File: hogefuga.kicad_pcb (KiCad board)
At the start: 2 copper layers, 95.3 x 97.6 mm, 45 parts, among them J1 MJ-4PP-9, SW1 SW_PUSH, SW10 SW_PUSH, SW11 SW_PUSH, SW12 SW_PUSH, SW13 SW_PUSH, SW14 SW_PUSH, SW15 SW_PUSH, SW16 SW_PUSH, SW17 SW_PUSH, SW18 SW_PUSH, SW19 SW_PUSH, SW2 SW_PUSH, SW20 SW_PUSH, SW3 SW_PUSH, SW4 SW_PUSH, SW5 SW_PUSH, SW6 SW_PUSH, SW7 SW_PUSH, SW8 SW_PUSH, SW9 SW_PUSH, U1 ProMicro

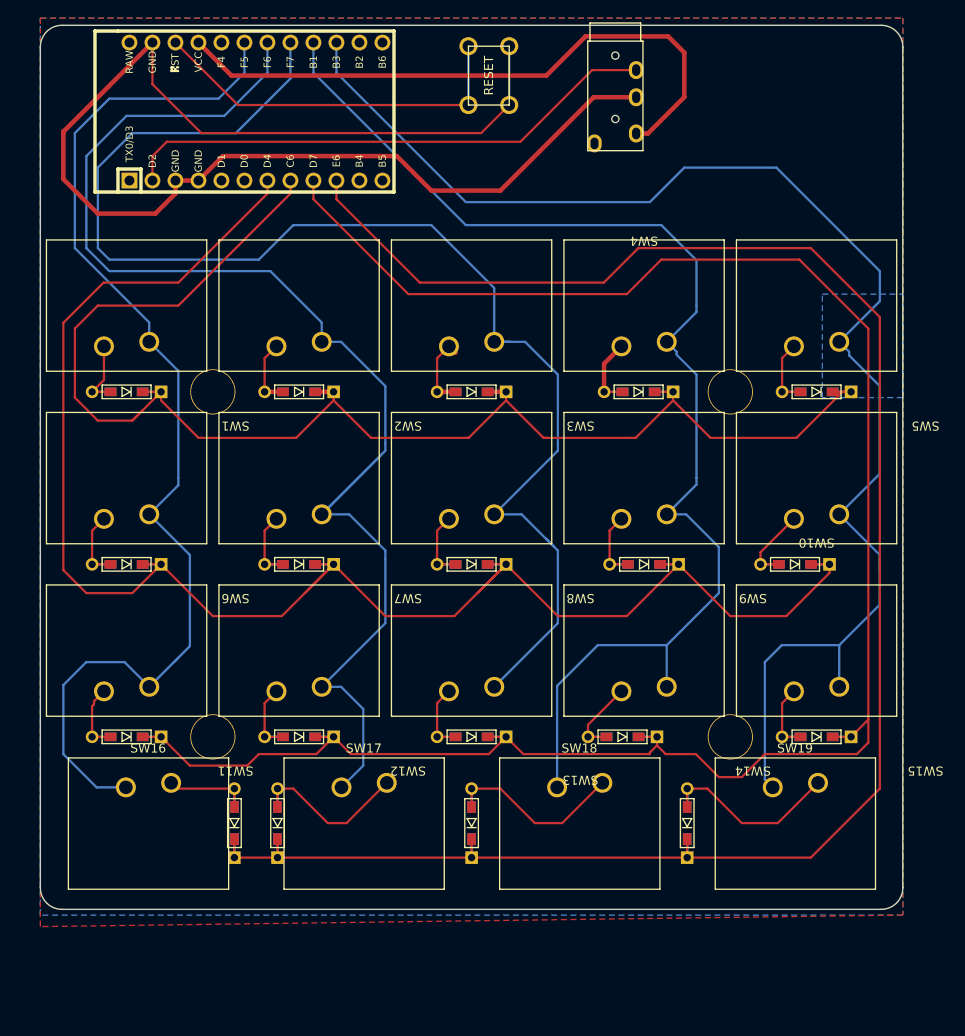
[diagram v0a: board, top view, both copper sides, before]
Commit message: rev0.2
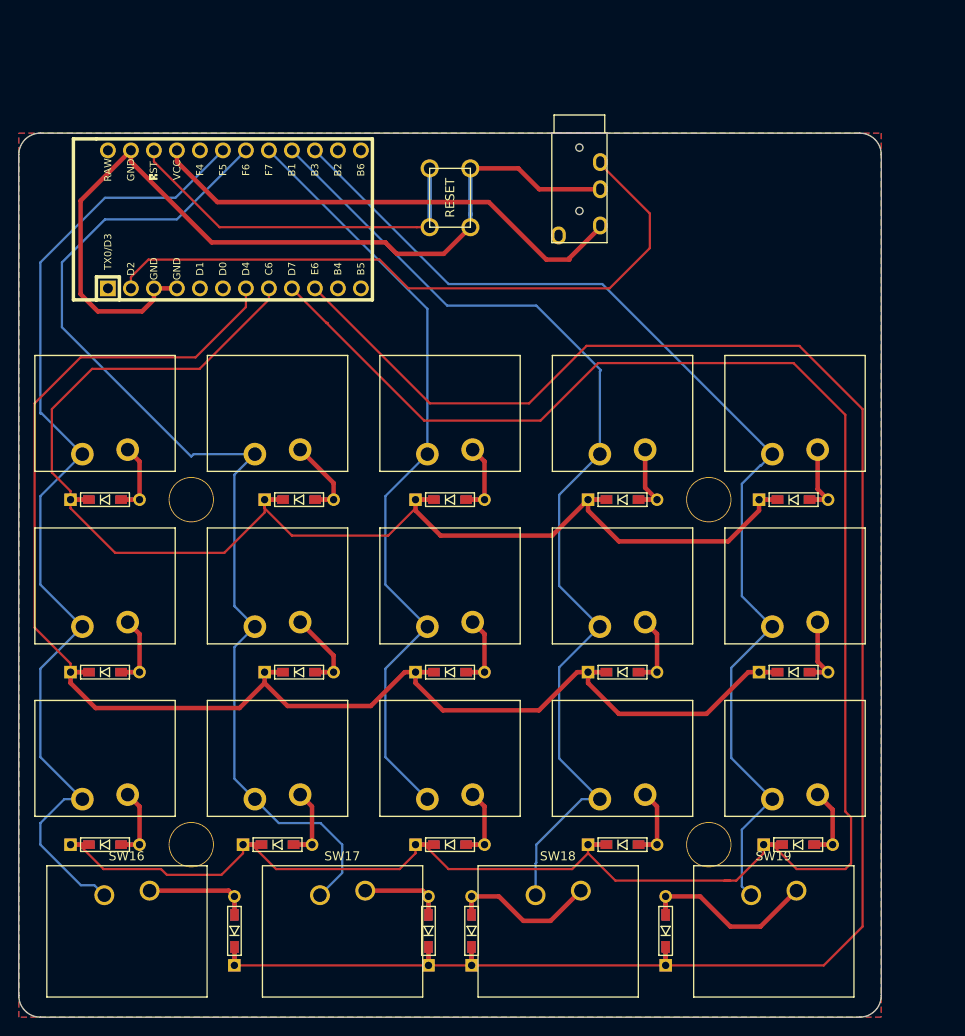
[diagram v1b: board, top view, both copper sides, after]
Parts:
- removed the Ref** at (133.3, 66.7)
- removed the Ref** at (133.3, 104.8)
- removed the Ref** at (76.2, 104.8)
- removed the Ref** at (76.2, 66.7)
- added Ref**: Val**, kbd:HOLE, F.Cu at (131.0, 78.6)
- added Ref**: Val**, kbd:HOLE, F.Cu at (131.0, 116.7)
- added Ref**: Val**, kbd:HOLE, F.Cu at (73.8, 116.7)
- added Ref**: Val**, kbd:HOLE, F.Cu at (73.8, 78.6)
- SW1, SW10, SW11, SW12, SW13, SW14, SW15, SW2, SW3, SW4, SW5, SW6, SW7, SW8, SW9: footprint lib:SW_Matias_1.00u -> keyboard_parts:ALPS_SKCM
- moved D17 20.5 mm to (100.0, 126.2)
- moved SW20 14.2 mm to (102.4, 45.2)
- moved D5 12.2 mm to (140.3, 78.6), turned to 0 degrees
- moved D13 12.1 mm to (102.4, 116.7), turned to 0 degrees
- moved D19 12.1 mm to (126.2, 126.2)
- moved D3 12.1 mm to (102.4, 78.6), turned to 0 degrees
- moved D8 12.1 mm to (102.4, 97.6), turned to 0 degrees
- moved D9 12.1 mm to (121.4, 97.6), turned to 0 degrees
- moved SW1 12.1 mm to (64.3, 69.1)
- moved SW10 12.1 mm to (140.5, 88.1)
- moved SW16 12.1 mm to (66.7, 126.2)
- moved SW17 12.1 mm to (90.5, 126.2)
- moved SW18 12.1 mm to (114.3, 126.2)
- moved SW2 12.1 mm to (83.3, 69.1)
- moved SW3 12.1 mm to (102.4, 69.1)
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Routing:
- net GND: track 161.6 -> 97.3 mm
- net col3: track 149.4 -> 86.6 mm
- net col5: track 155.2 -> 121.6 mm
- net col2: track 146.1 -> 120.1 mm
- net col4: track 136.6 -> 113.8 mm
- net row1: track 193.0 -> 173.5 mm
- net VCC: track 69.6 -> 54.2 mm
- net row2: track 228.7 -> 243.0 mm
- net data: track 60.1 -> 74.3 mm
- net col1: track 124.2 -> 111.8 mm
- net row0: track 167.0 -> 157.3 mm
- net Net-(D17-Pad2): track 19.6 -> 11.3 mm
- net Net-(D18-Pad2): track 21.9 -> 18.6 mm
- net row3: track 213.4 -> 215.8 mm
- net Net-(D16-Pad2): track 11.3 -> 13.7 mm
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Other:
- outline, holes or cut-outs redrawn
- board text added: "hogefuga keyboard v0.2 by yswallow"
- board text removed: "hogefuga v0.1 by yswallow"
